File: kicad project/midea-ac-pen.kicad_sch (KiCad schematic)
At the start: 9 parts, among them J1 Conn_01x08_Pin, J2 Conn_01x08_Pin, J3 USB_A, Q1 2N3904, Q2 2N3904

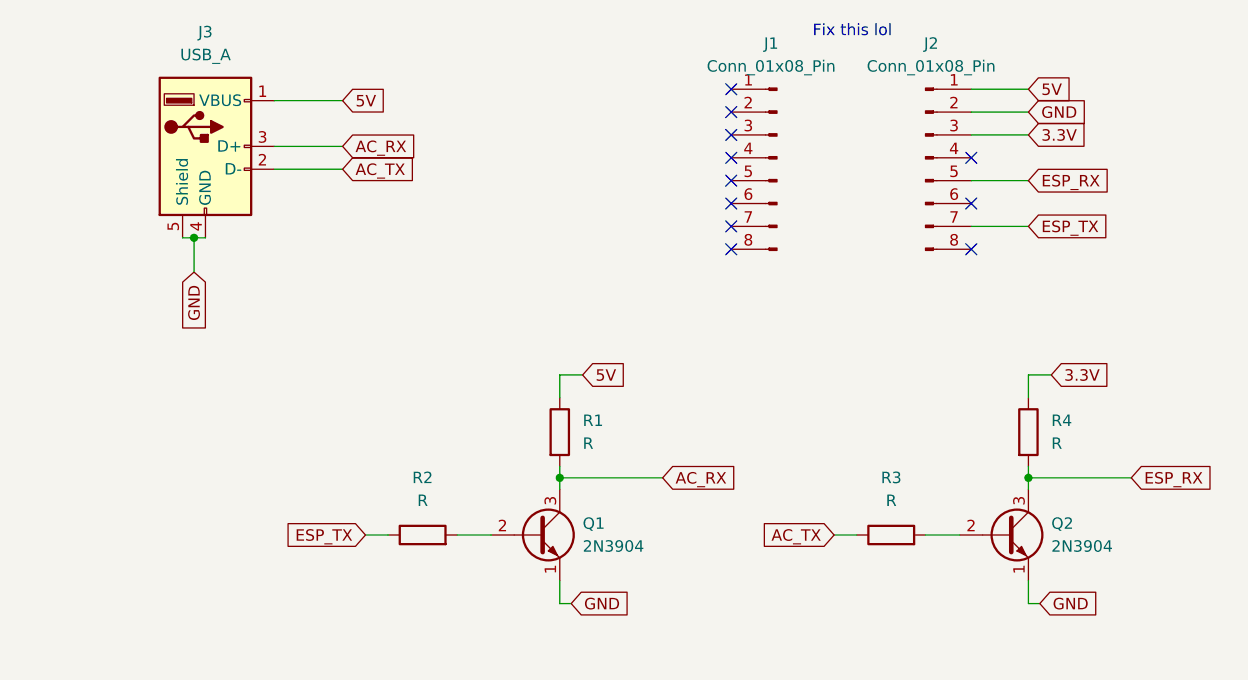
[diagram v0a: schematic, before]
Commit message: draw pcb
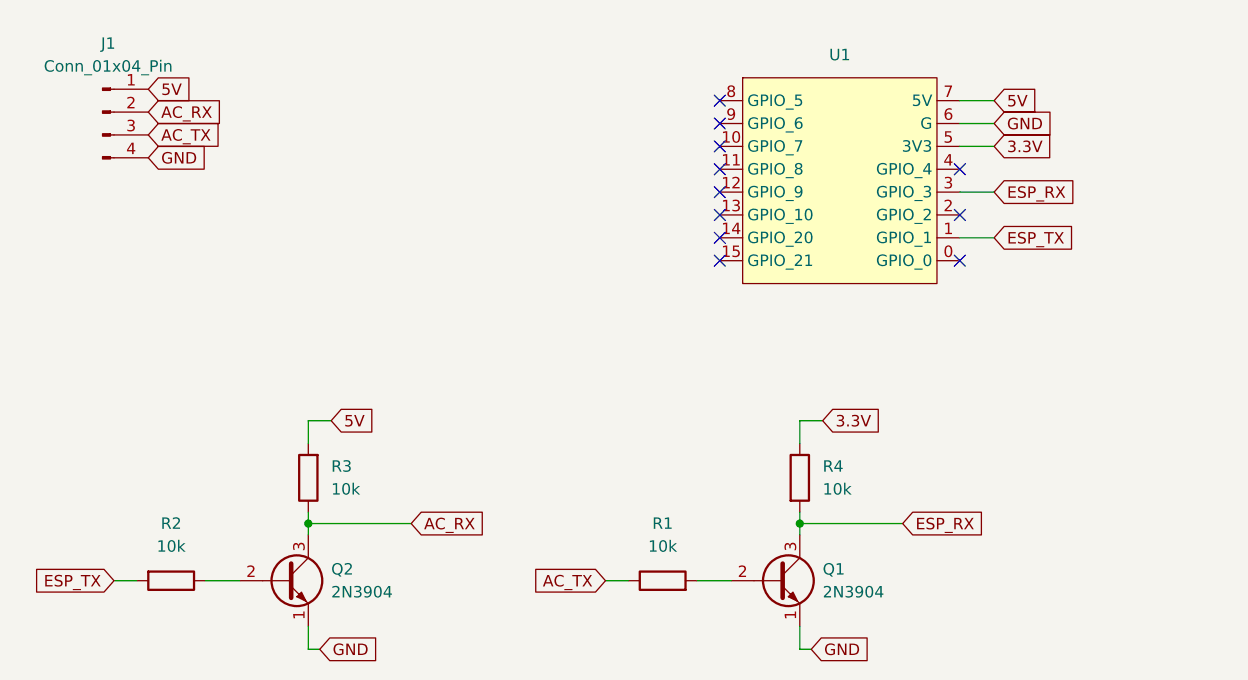
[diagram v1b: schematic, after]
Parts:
- removed J1, J2: Conn_01x08_Pin, symbol Connector:Conn_01x08_Pin
- removed J3: USB_A, symbol Connector:USB_A
- added J1: Conn_01x04_Pin, ESP32_C3_Super_Mini:PCB_USB, symbol Connector:Conn_01x04_Pin
- added U1: ~, ESP32_C3_Super_Mini:ESP32_C3_Super_Mini, symbol ESP32_C3_Super_Mini:ESP32_C3_Super_Mini
- Q1: renamed from Q2; footprint (none) -> Package_TO_SOT_THT:TO-92
- Q2: renamed from Q1; footprint (none) -> Package_TO_SOT_THT:TO-92
- R1: renamed from R3; value R -> 10k; footprint (none) -> Resistor_THT:R_Axial_DIN0204_L3.6mm_D1.6mm_P2.54mm_Vertical
- R2, R4: value R -> 10k; footprint (none) -> Resistor_THT:R_Axial_DIN0204_L3.6mm_D1.6mm_P2.54mm_Vertical
- R3: renamed from R1; value R -> 10k; footprint (none) -> Resistor_THT:R_Axial_DIN0204_L3.6mm_D1.6mm_P2.54mm_Vertical
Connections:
- net 3.3V: now also U1.5 (3V3)
- net 5V: now also R3.2, J1.1 (Pin_1), U1.7 (5V); no longer R3.1
- net AC_RX: now also R3.1, J1.2 (Pin_2); no longer R3.2
- net AC_TX: now also J1.3 (Pin_3)
- net ESP_RX: now also U1.3 (GPIO_3)
- net ESP_TX: now also R2.2, U1.1 (GPIO_1); no longer R2.1
- net GND: now also J1.4 (Pin_4), U1.6 (G)
- net at Q2.2 (B): now also R2.1; no longer R2.2
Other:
- note removed: "Fix this lol"
- moved on the sheet: Q1, Q2, R1, R2, R3, R4
